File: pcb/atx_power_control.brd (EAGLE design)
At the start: 100 x 70 mm, 45 parts, among them IC2 REG1117, IC3 STM32F042F4, IC4 MY_7905DT, J1 ATX24RH, SW3 324_SW, SW4 324_SW, U2 USBC_16P

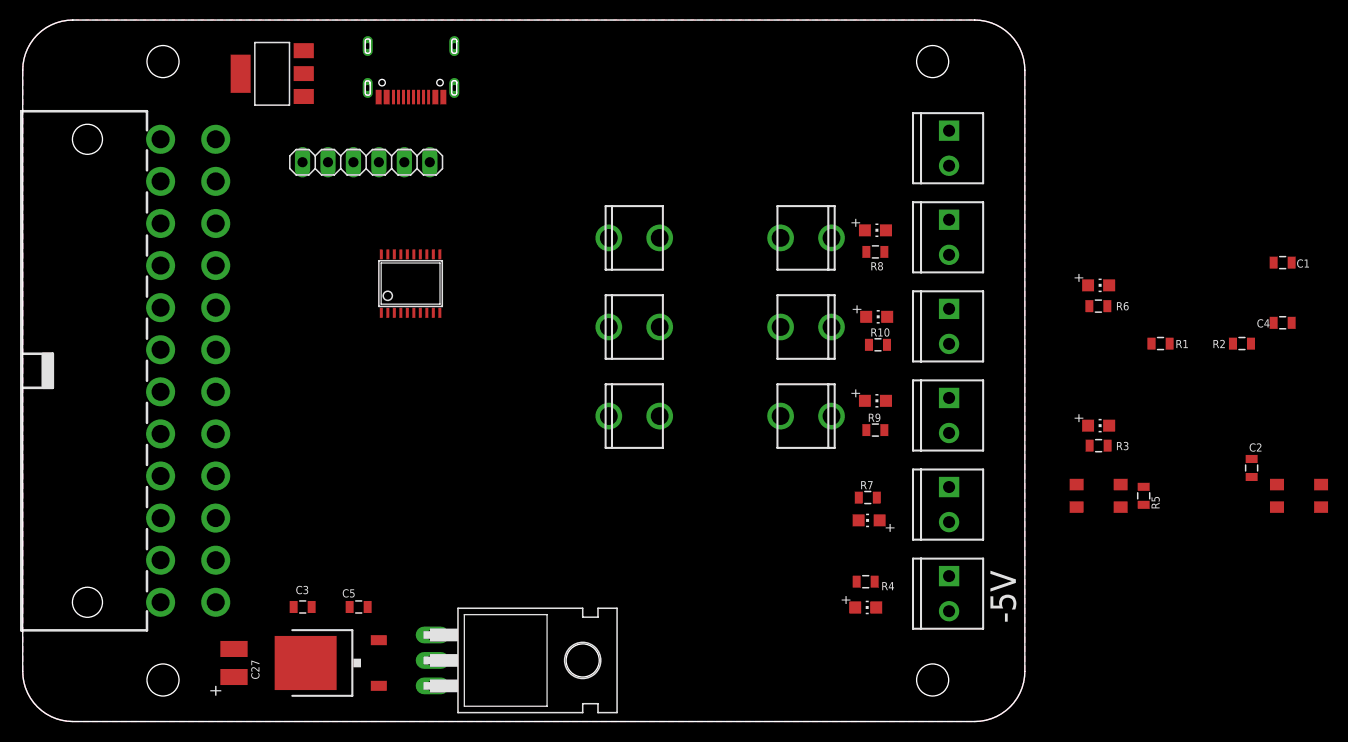
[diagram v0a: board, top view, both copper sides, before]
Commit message: working on PCB
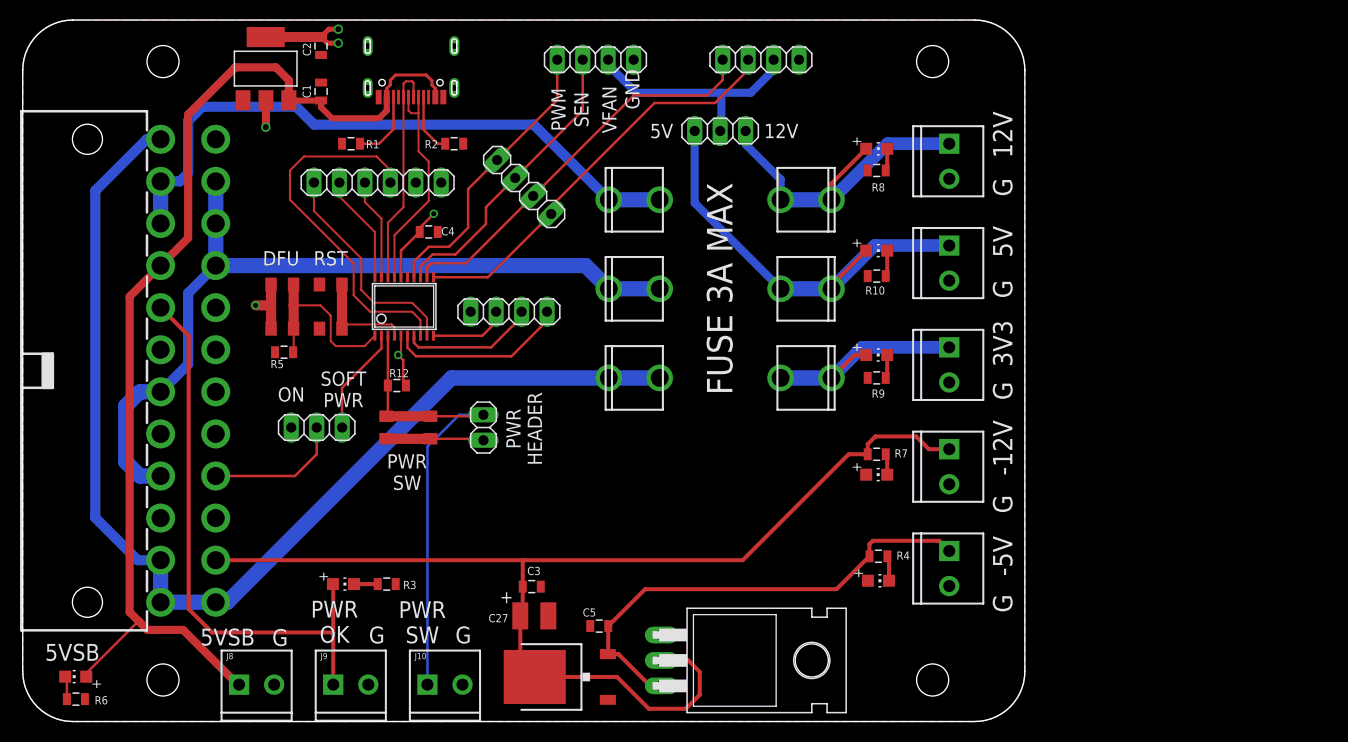
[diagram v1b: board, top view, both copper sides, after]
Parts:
- removed J5: (no value), SparkFun-Connectors:SCREWTERMINAL-3.5MM-2
- added J10, J8, J9: (no value), SparkFun-Connectors:SCREWTERMINAL-3.5MM-2
- added JP1, JP2, JP7, JP8: (no value), pinhead:1X04
- added JP4, JP5: (no value), pinhead:1X03
- added JP6: (no value), pinhead:1X02
- added R12: 5.1K, joyAnalog:0805
- added SW1: 324_SW, 3pos_slide_switch_centered:342_SWICH_FOOT
- R8: value 1K -> 5K
- moved R6 109.3 mm to (5.31, 2.24), turned to 180 degrees
- moved LED2 109.3 mm to (5.29, 4.48), turned to 90 degrees
- moved C2 102.0 mm to (29.8, 67.4), turned to 90 degrees
- moved SW3 98.5 mm to (30.7, 41.4), turned to 270 degrees
- moved C1 97.5 mm to (29.8, 62.9), turned to 270 degrees
- moved R5 87.0 mm to (26.1, 36.9), turned to 0 degrees
- moved C4 85.7 mm to (40.5, 48.9), turned to 180 degrees
- moved SW4 83.6 mm to (25.9, 41.4), turned to 270 degrees
- moved R1 83.2 mm to (32.8, 57.7)
- moved R2 81.1 mm to (43.1, 57.7)
- moved LED3 77.0 mm to (32.0, 13.7)
- moved R3 72.4 mm to (36.3, 13.7), turned to 180 degrees
- moved C27 30.3 mm to (51.1, 10.5), turned to 0 degrees
- moved C5 24.1 mm to (57.5, 9.53)
- moved C3 23.0 mm to (50.8, 13.5)
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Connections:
- new net N$17: JP1.2, JP2.2, JP4.2
- new net N$19: F3.3, F3.4, J2.1, LED6.A
- new net N$21: IC3.12, JP1.4, JP7.3
- new net N$22: IC3.13, JP2.3, JP7.2
- new net N$23: IC3.14, JP2.4, JP7.1
- new net N$24: IC3.2, JP5.1
- new net N$25: J1.16, JP5.2
- new net N$26: IC3.3, J10.1, JP6.1, R12.1, SW1.P$2, SW1.P$3
- new net N$27: IC3.6, JP8.4
- new net N$28: J1.8, J9.1, LED3.A
- new net N$30: IC3.7, JP8.3
- new net N$32: IC3.10, JP8.2
- net +3V3: now also R12.2; no longer LED2.A, LED3.A
- net GND: now also J10.2, J2.2, J3.2, J4.2, J6.2, J7.2, J8.2, J9.2, JP1.1, JP2.1, JP5.3, JP6.2, JP8.1, R3.1, SW1.P$1, SW1.P$4; no longer J5.1, J5.2
- net N$11: no longer J4.2
- net N$14: now also IC3.11, JP1.3, JP7.4; no longer F2.1, F2.2, J6.1, J6.2, LED5.A
- net N$15: now also JP4.1; no longer J7.2
- net N$16: now also F2.1, F2.2, J6.1, JP4.3, LED5.A; no longer F3.3, F3.4, J2.1, J2.2, LED6.A
- net N$2: no longer J3.2
- net VCC: now also J8.1, LED2.A
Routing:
- net N$2: track 0.00 -> 116.7 mm
- net N$12: track 0.00 -> 112.8 mm
- net VCC: track 0.00 -> 109.0 mm
- net N$10: track 0.00 -> 82.2 mm
- net N$13: track 0.00 -> 64.0 mm
- net N$28: track 0.00 -> 56.7 mm
- net N$26: track 0.00 -> 48.7 mm
- net N$11: track 0.00 -> 48.2 mm
- net N$15: track 0.00 -> 43.2 mm
- net N$14: track 0.00 -> 41.4 mm
- net N$21: track 0.00 -> 40.3 mm
- net N$6: track 0.00 -> 36.7 mm
- net N$16: track 0.00 -> 34.0 mm
- net +3V3: track 0.00 -> 31.3 mm, vias 0 -> 6
- net N$22: track 0.00 -> 29.7 mm
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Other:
- board text added: "-12V"
- board text added: "12V"
- board text added: "5V"
- board text added: "5VSB"
- board text added: "DFU"
- board text added: "FUSE 3A MAX"
- board text added: "GND"
- board text added: "ON"
- board text added: "PWM"
- board text added: "PWR HEADER"
- board text added: "PWR OK"
- board text added: "PWR SW"
- board text added: "RST"
- board text added: "SEN"
- board text added: "SOFT PWR"
- board text added: "VFAN"
- board text removed: "CLK"
- board text removed: "DIO"
- board text removed: "RX"
- board text removed: "TX"
